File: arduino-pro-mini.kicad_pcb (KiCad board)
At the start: 2 copper layers, 17.8 x 33 mm, 21 parts, among them Q1 Resonator, U1 ATMEGA328-A, U2 MIC5205

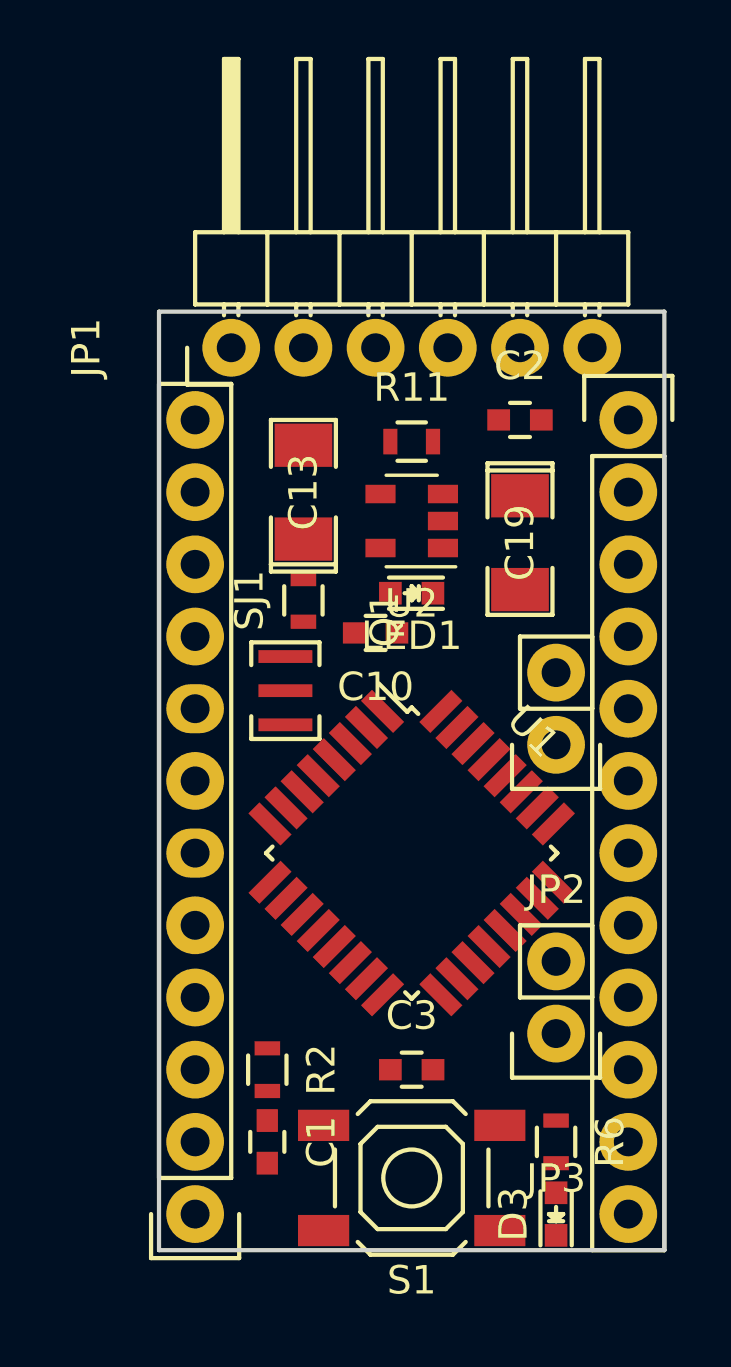
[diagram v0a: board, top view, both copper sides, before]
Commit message: update
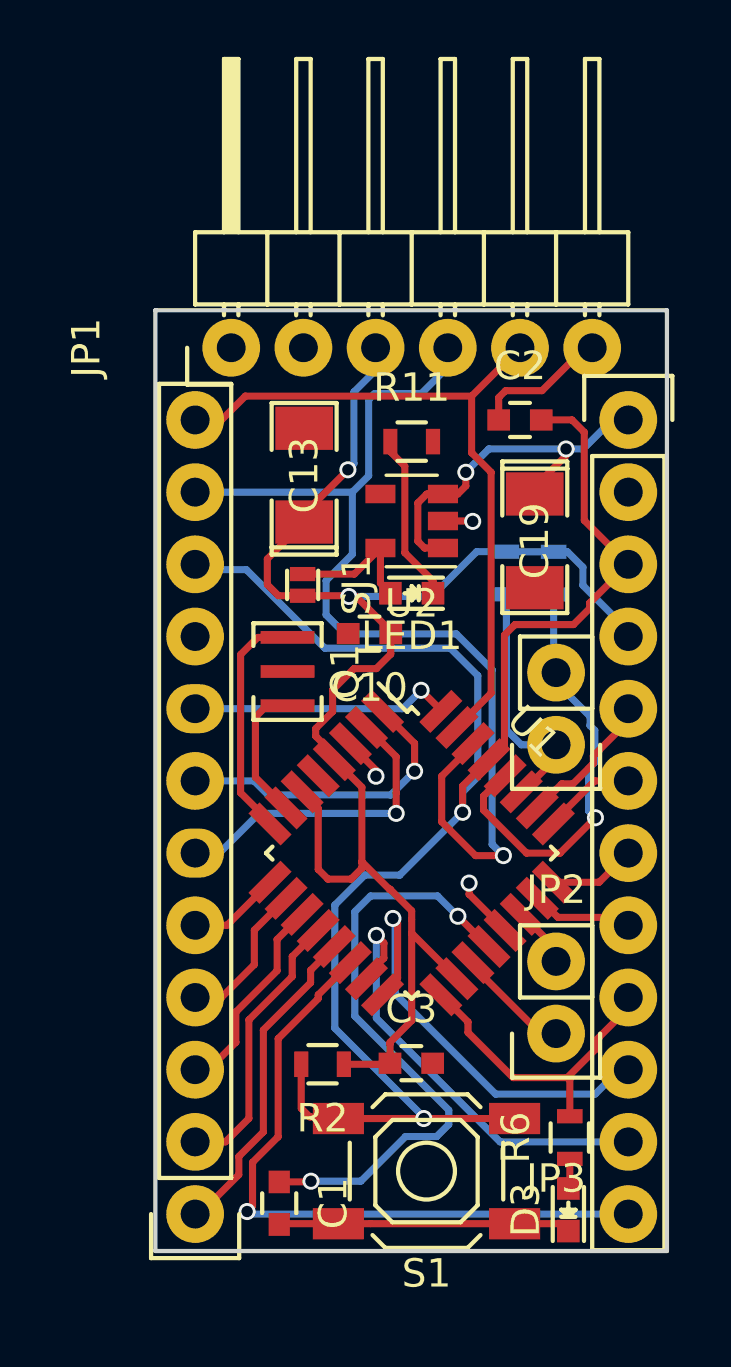
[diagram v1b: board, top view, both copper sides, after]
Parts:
- added R1: R, Resistors_SMD:R_0603, B.Cu at (126.3, 94.4)
- added R3: R, Resistors_SMD:R_0603, B.Cu at (128.0, 94.4)
- SJ1: footprint Resistors_SMD:R_0603 -> arduino-pro-mini:jumper
- moved C1 2.20 mm to (118.3, 116.6)
- moved R2 1.95 mm to (119.8, 111.7), turned to 180 degrees
- moved Q1 0.68 mm to (118.6, 97.9)
- moved C13 0.60 mm to (119.2, 91.0)
- moved S1 0.57 mm to (123.5, 115.5)
- moved SJ1 0.55 mm to (119.1, 94.9), turned to 270 degrees
- moved C19 0.52 mm to (127.3, 93.3)
- moved R6 0.51 mm to (128.5, 114.3), turned to 90 degrees
- moved D3 0.46 mm to (128.5, 116.8)
- moved C3 0.23 mm to (122.9, 111.7)
- moved C10 0.22 mm to (121.5, 96.6)
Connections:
- JP1 pad 1: DTR -> GND
- JP1 pad 2: TXO -> GND
- JP1 pad 3: RXI -> VCC
- JP1 pad 4: VCC -> RXI
- JP1 pad 5: GND -> TXO
- JP1 pad 6: GND -> DTR
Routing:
- net RESET: track 0.00 -> 59.8 mm, vias 0 -> 2
- net VCC: track 0.00 -> 54.8 mm, vias 0 -> 2
- net RXI: track 0.00 -> 36.9 mm, vias 0 -> 1
- net TXO: track 0.00 -> 24.9 mm
- net D10: track 0.00 -> 24.0 mm, vias 0 -> 1
- net Net-(C1-Pad1): track 0.00 -> 21.3 mm, vias 0 -> 2
- net MISO: track 0.00 -> 15.7 mm, vias 0 -> 1
- net MOSI: track 0.00 -> 15.6 mm, vias 0 -> 1
- net A5: track 0.00 -> 15.3 mm, vias 0 -> 1
- net GND: track 0.00 -> 15.1 mm, vias 0 -> 3
- net RAW: track 0.00 -> 13.3 mm, vias 0 -> 2
- net D9: track 0.00 -> 11.8 mm
- net D4: track 0.00 -> 11.1 mm, vias 0 -> 1
- net SCK: track 0.00 -> 11.0 mm
- net D3: track 0.00 -> 10.8 mm, vias 0 -> 1
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- added copper zone on B.Cu, net GND
- added copper zone on F.Cu, net GND
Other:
- board size 17.8 x 33 mm -> 18 x 33.1 mm
